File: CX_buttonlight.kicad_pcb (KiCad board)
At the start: 2 copper layers, 17 x 5.5 mm, 10 parts, among them U1 LM317L_SOT-89

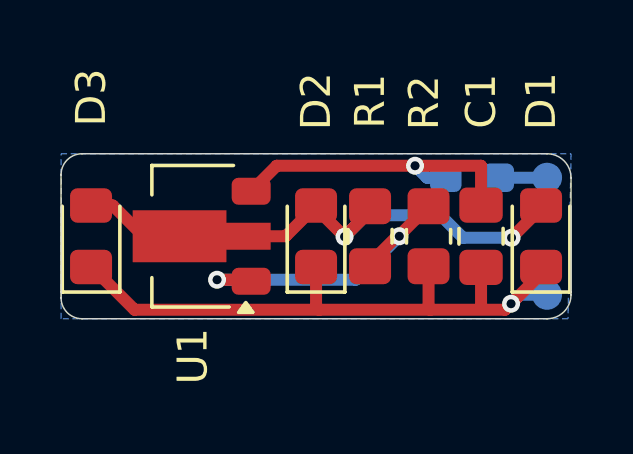
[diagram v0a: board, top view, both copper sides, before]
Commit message: updated design (tweaks + specs), sent to JLCPCB
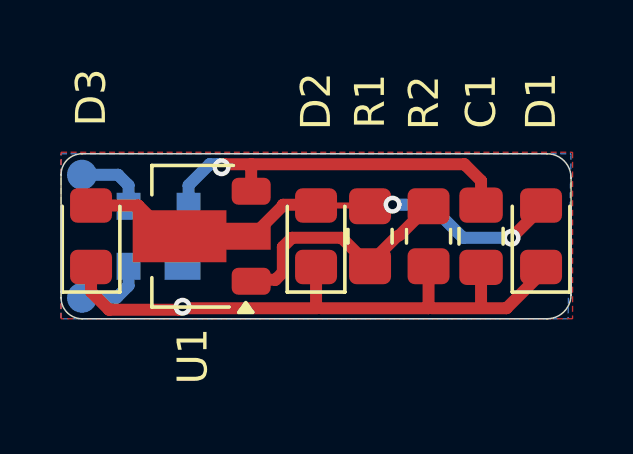
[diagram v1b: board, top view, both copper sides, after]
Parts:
- D4: value D -> BAS4002ARPPE6327HTSA1; footprint Diode_SMD:D_0603_1608Metric_Pad1.05x0.95mm_HandSolder -> EC-parts:BAS4002ARPPE6327HTSA1
- moved Ground1 16.0 mm to (100.7, 60.7)
- moved Supply1 16.0 mm to (100.7, 64.8)
- moved D4 10.6 mm to (103.2, 62.8), turned to 180 degrees
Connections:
- C1 pad 1: Net-(D4-K) -> Net-(D4-+)
- D4 pad 1: Net-(D4-K) -> GND
- Ground1 pad 1: GND -> Net-(D4-~_2)
- U1 pad 3: Net-(D4-K) -> Net-(D4-+)
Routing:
- net Net-(D4-+): track 0.00 -> 13.0 mm, vias 0 -> 1
- net Net-(D4-K): track 10.5 -> 0.00 mm, vias 1 -> 0
- net Net-(D4-~_2): track 0.00 -> 2.39 mm
- net Net-(U1-ADJ): track 10.7 -> 8.45 mm, vias 2 -> 0
- net Net-(D1-A): track 18.5 -> 16.8 mm
- net GND: track 21.9 -> 21.0 mm
- net Net-(D4-~_1): track 1.62 -> 2.37 mm
- added copper zone on B.Cu, net GND
- added copper zone on F.Cu, net Net-(D1-A)
- removed copper zone on B.Cu, net (none)
